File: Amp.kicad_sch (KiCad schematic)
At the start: 28 parts

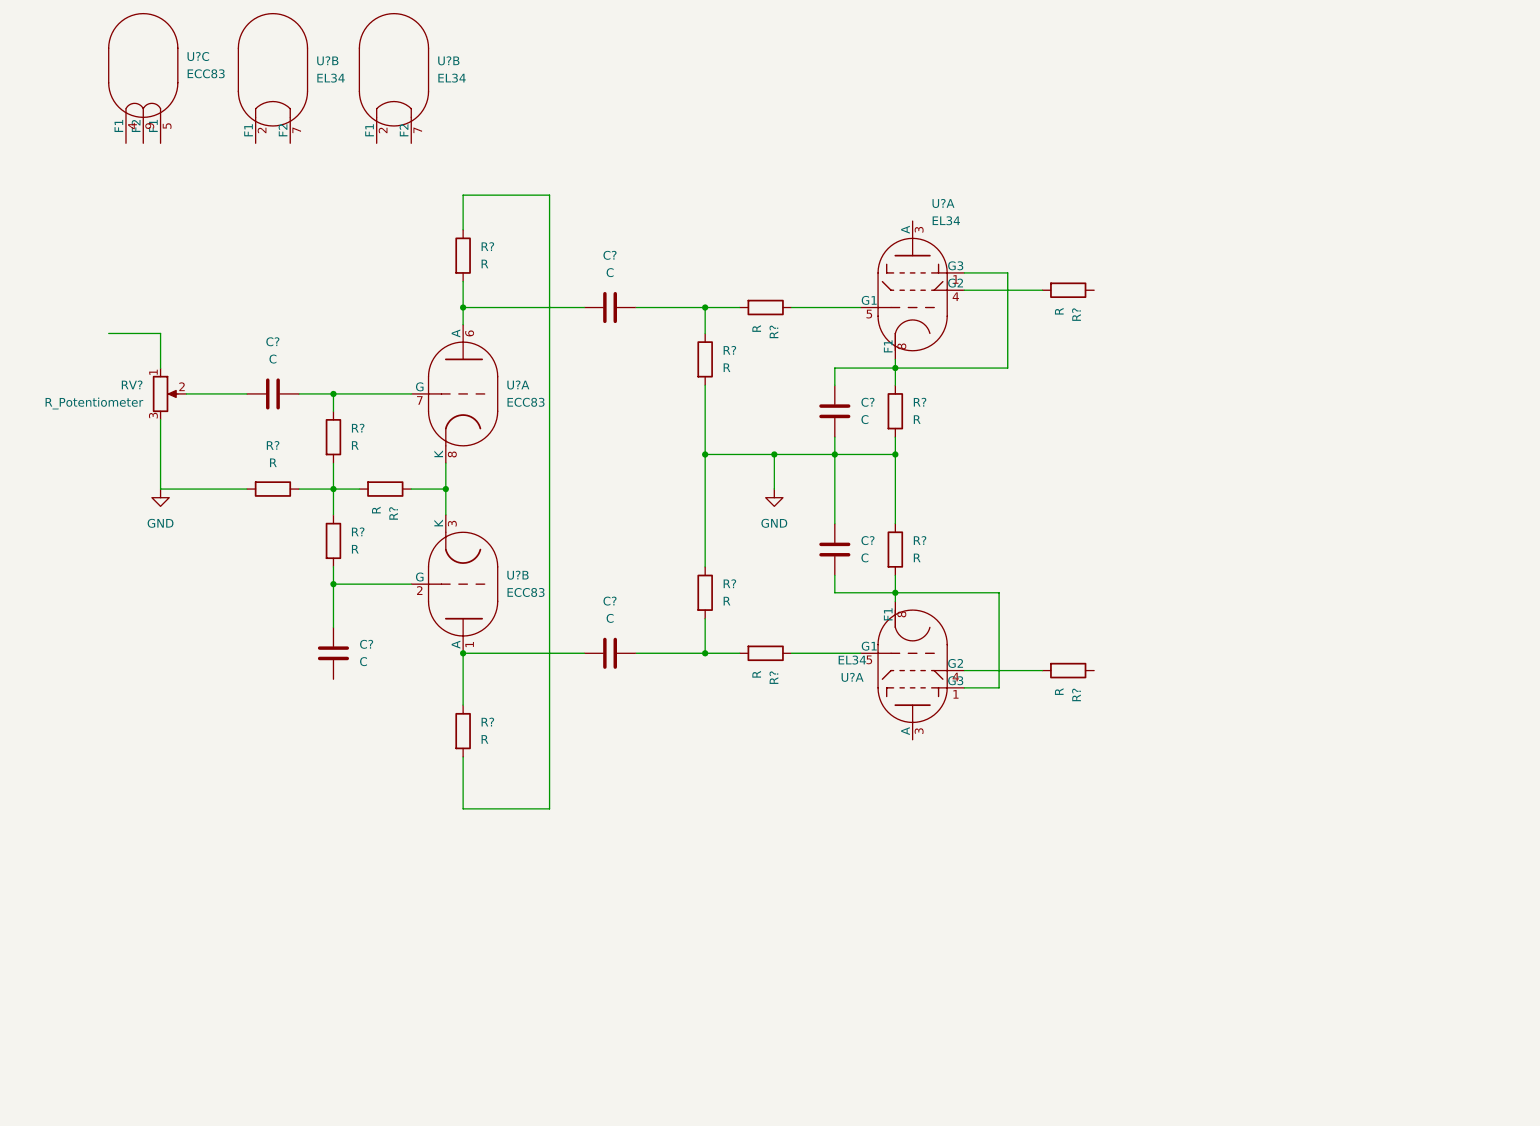
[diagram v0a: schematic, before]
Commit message: Some updates
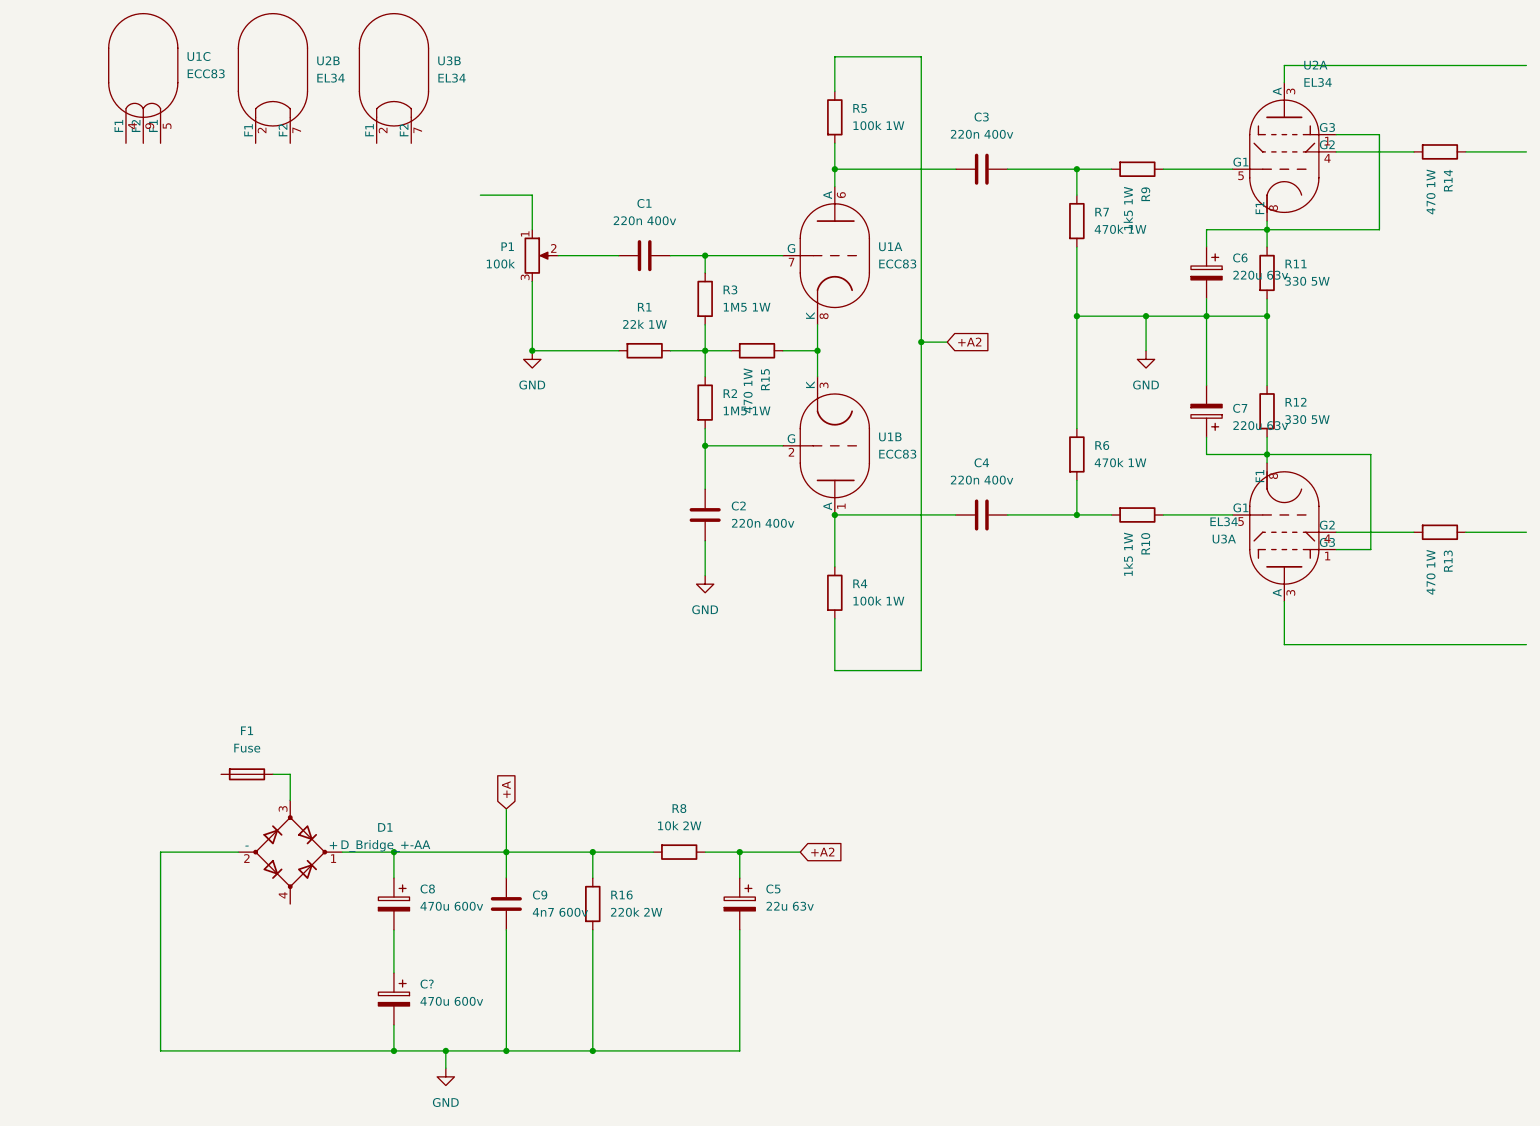
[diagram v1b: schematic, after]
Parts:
- added C5: 22u 63v, Capacitor_THT:CP_Radial_D6.3mm_P2.50mm, symbol Device:C_Polarized
- added C8, C?: 470u 600v, Capacitor_THT:CP_Radial_D40.0mm_P10.00mm_SnapIn, symbol Device:C_Polarized
- added C9: 4n7 600v, Capacitor_THT:C_Rect_L16.5mm_W5.0mm_P15.00mm_MKT, symbol Device:C
- added D1: D_Bridge_+-AA, Diode_THT:Diode_Bridge_32.0x5.6x17.0mm_P10.0mm_P7.5mm, symbol Device:D_Bridge_+-AA
- added F1: Fuse, symbol Device:Fuse
- added R16: 220k 2W, Resistor_THT:R_Axial_DIN0516_L15.5mm_D5.0mm_P20.32mm_Horizontal, symbol Device:R
- added R8: 10k 2W, symbol Device:R
- C1, C3, C4: renamed from C?; value C -> 220n 400v; footprint (none) -> Capacitor_THT:C_Rect_L16.5mm_W5.0mm_P15.00mm_MKT
- C2: renamed from C?; value C -> 220n 400v
- C6, C7: renamed from C?; value C -> 220u 63v; footprint (none) -> Capacitor_THT:C_Radial_D10.0mm_H16.0mm_P5.00mm; symbol Device:C -> Device:C_Polarized
- P1: renamed from RV?; value R_Potentiometer -> 100k; footprint (none) -> Potentiometer_THT:Potentiometer_TT_P0915N
- R1: renamed from R?; value R -> 22k 1W; footprint (none) -> Resistor_THT:R_Axial_DIN0414_L11.9mm_D4.5mm_P20.32mm_Horizontal
- R10, R9: renamed from R?; value R -> 1k5 1W; footprint (none) -> Resistor_THT:R_Axial_DIN0414_L11.9mm_D4.5mm_P20.32mm_Horizontal
- R11, R12: renamed from R?; value R -> 330 5W; footprint (none) -> Resistor_THT:R_Axial_Power_L25.0mm_W6.4mm_P30.48mm
- R13, R14, R15: renamed from R?; value R -> 470 1W; footprint (none) -> Resistor_THT:R_Axial_DIN0414_L11.9mm_D4.5mm_P20.32mm_Horizontal
- R2, R3: renamed from R?; value R -> 1M5 1W; footprint (none) -> Resistor_THT:R_Axial_DIN0414_L11.9mm_D4.5mm_P20.32mm_Horizontal
- R4, R5: renamed from R?; value R -> 100k 1W; footprint (none) -> Resistor_THT:R_Axial_DIN0414_L11.9mm_D4.5mm_P20.32mm_Horizontal
- R6, R7: renamed from R?; value R -> 470k 1W; footprint (none) -> Resistor_THT:R_Axial_DIN0414_L11.9mm_D4.5mm_P20.32mm_Horizontal
- gave numbers to parts that had none: 3
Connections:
- net GND: now also C2.1, C6.2, C5.2, C9.1, C?.2, D1.2 (-), R16.2; no longer C6.1
- net at R11.1, U2.1 (G3), U2.8 (F1): now also C6.1; no longer C6.2
- net +A2: now reaches R4.2, R5.1
- net +A2: now also C5.1, R8.1
- new net: C8.2, C?.1
- new net: D1.3, F1.1
- new net +A: C8.1, C9.2, D1.1 (+), R16.1, R8.2
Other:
- moved on the sheet: C1, C2, C3, C4, P1, R1, R10, R11, R12, R13, R14, R15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
